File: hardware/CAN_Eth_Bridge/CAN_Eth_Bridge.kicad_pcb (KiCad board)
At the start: 2 copper layers, 22.6 x 85 mm, 72 parts, among them J101 Conn_01x05_Pin, J102 Global LV and CAN, J301 RJ45_Amphenol_RJMG1BD3B8K1ANR, Q301 MMBT5550L, Q302 MMBT5550L, SW102 SW_DIP_x06, U101 MCP2542FDxMF, U102 AP7384-50SA, U103 XMSM0G3507SDGS28R, U104 AP7381-33SA-7, U301 W5500, Y301 Crystal_GND24

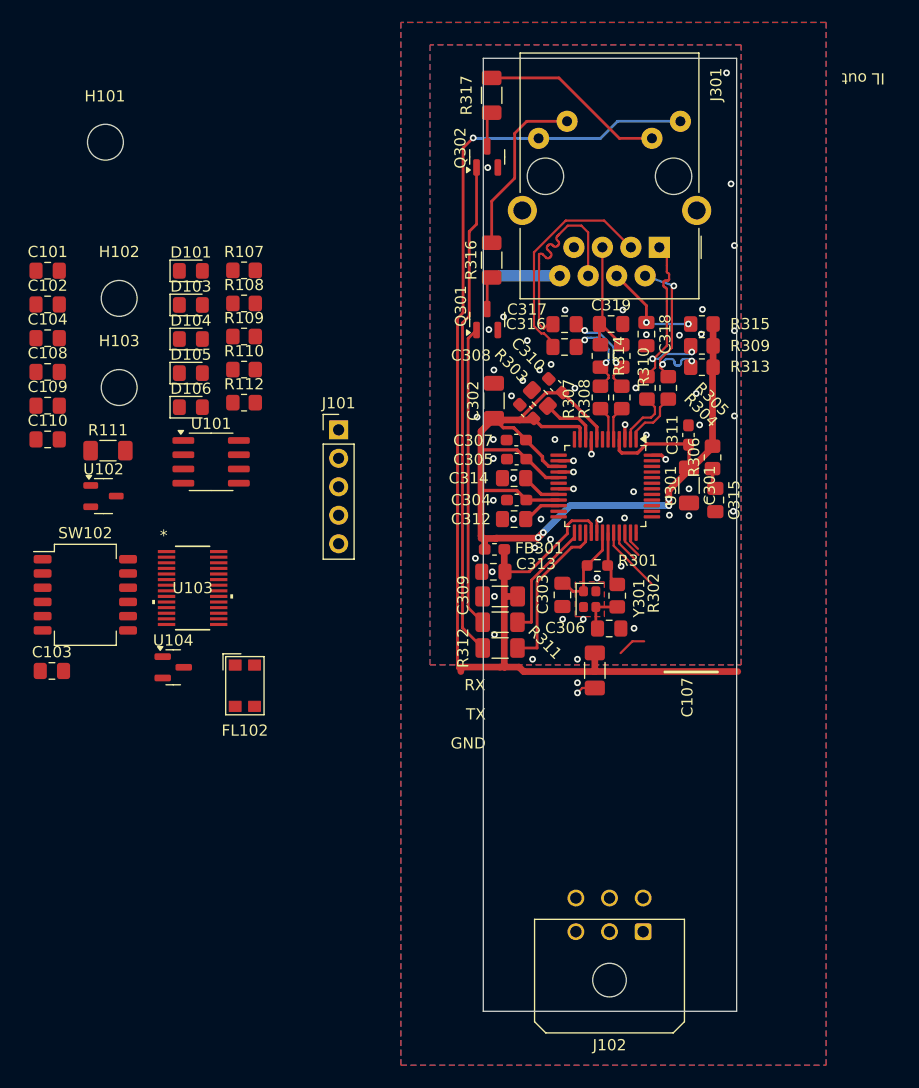
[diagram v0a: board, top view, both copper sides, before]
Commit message: hdd failure D:
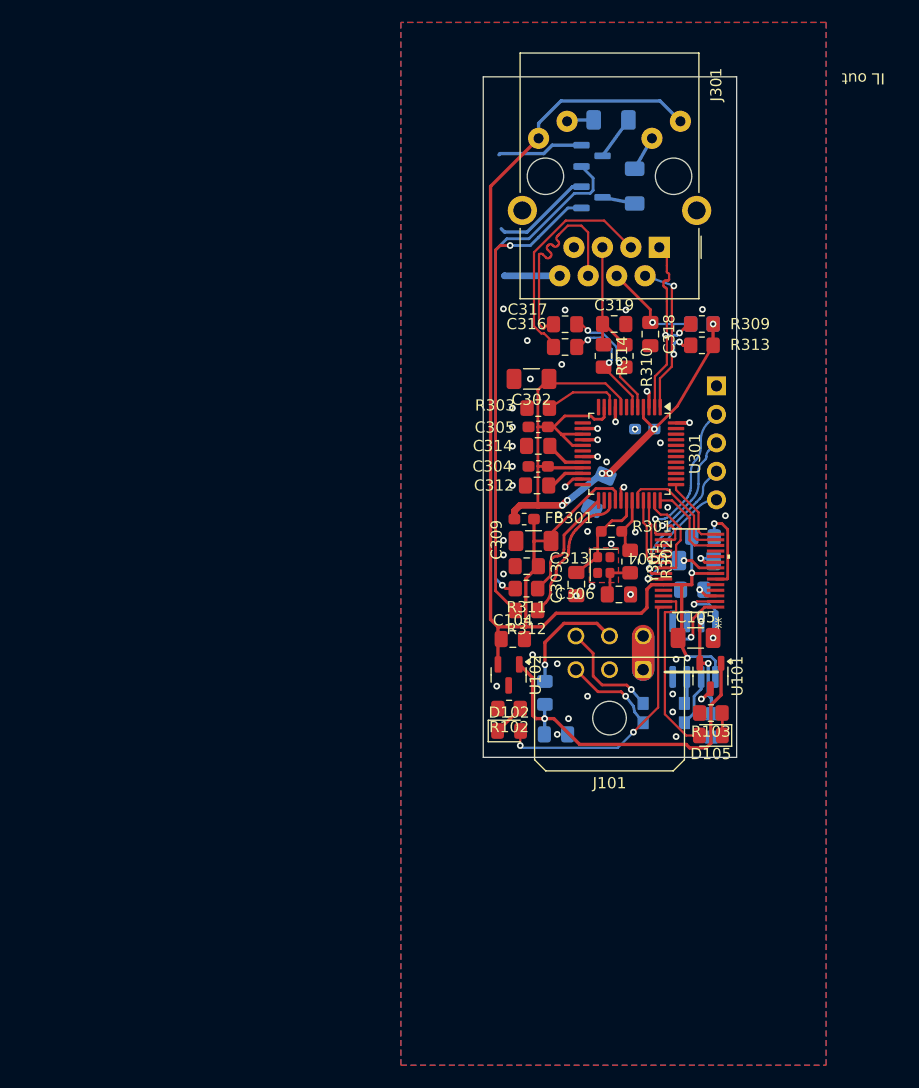
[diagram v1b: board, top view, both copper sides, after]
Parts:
- removed C102, C108, C109, C110, C315: 220n, Capacitor_SMD:C_0805_2012Metric_Pad1.18x1.45mm_HandSolder
- removed C107: 10u, Capacitor_SMD:C_1206_3216Metric_Pad1.33x1.80mm_HandSolder
- removed C307, C308, C310: 100n, Capacitor_SMD:C_0603_1608Metric_Pad1.08x0.95mm_HandSolder
- removed D103, D104: yellow, LED_SMD:LED_0805_2012Metric_Pad1.15x1.40mm_HandSolder
- removed D106: blue, LED_SMD:LED_0805_2012Metric_Pad1.15x1.40mm_HandSolder
- removed FL102: Choke_CommonMode_FerriteCore_1243, Inductor_SMD:L_CommonModeChoke_Coilcraft_1812CAN
- removed H101, H102, H103: MountingHole, MountingHole:MountingHole_3.2mm_M3
- removed R107, R108, R109: 2.4k, Resistor_SMD:R_0805_2012Metric_Pad1.20x1.40mm_HandSolder
- removed R110: 3.32k, Resistor_SMD:R_0805_2012Metric_Pad1.20x1.40mm_HandSolder
- removed R111: 100k, Resistor_SMD:R_1206_3216Metric_Pad1.30x1.75mm_HandSolder
- removed R112: 40.2k, Resistor_SMD:R_0805_2012Metric_Pad1.20x1.40mm_HandSolder
- removed R304, R305, R307, R308: 14.3, Resistor_SMD:R_0805_2012Metric_Pad1.20x1.40mm_HandSolder
- removed R306: 10, Resistor_SMD:R_0805_2012Metric_Pad1.20x1.40mm_HandSolder
- removed SW102: SW_DIP_x06, Button_Switch_SMD:SW_DIP_SPSTx06_Slide_Copal_CHS-06B_W7.62mm_P1.27mm
- added C105: 10u, Capacitor_SMD:C_1206_3216Metric_Pad1.33x1.80mm_HandSolder, F.Cu at (152.3, 111.7)
- added C106: 220n, Capacitor_SMD:C_0805_2012Metric_Pad1.18x1.45mm_HandSolder, B.Cu at (152.0, 107.4)
- added D102: green, LED_SMD:LED_0805_2012Metric_Pad1.15x1.40mm_HandSolder, F.Cu at (135.7, 120.0)
- added FL101: Choke_CommonMode_FerriteCore_1243, Inductor_SMD:L_CommonModeChoke_Coilcraft_1812CAN, B.Cu at (149.5, 118.4)
- added R102: 2.4k, Resistor_SMD:R_0805_2012Metric_Pad1.20x1.40mm_HandSolder, F.Cu at (135.7, 118.0)
- added R103: 2.4k, Resistor_SMD:R_0805_2012Metric_Pad1.20x1.40mm_HandSolder, F.Cu at (153.7, 118.4)
- added R104: 2.4k, Resistor_SMD:R_0805_2012Metric_Pad1.20x1.40mm_HandSolder, B.Cu at (153.0, 102.7)
- added R105: 100k, Resistor_SMD:R_1206_3216Metric_Pad1.30x1.75mm_HandSolder, B.Cu at (152.4, 104.8)
- C101, C103, C301, C311, D101, Q301, Q302, R315, R316, R317: moved to B.Cu
- D105: value red -> blue
- J101: value Conn_01x05_Pin -> Global LV and CAN; footprint Connector_PinHeader_2.54mm:PinHeader_1x05_P2.54mm_Vertical -> Connector_Molex:Molex_Micro-Fit_3.0_43045-0600_2x03_P3.00mm_Horizontal
- J102: value Global LV and CAN -> Conn_01x05_Pin; footprint Connector_Molex:Molex_Micro-Fit_3.0_43045-0600_2x03_P3.00mm_Horizontal -> Connector_PinHeader_2.54mm:PinHeader_1x05_P2.54mm_Vertical; moved to B.Cu
- R311, R312: value 4.99k -> 3.32k; footprint Resistor_SMD:R_1206_3216Metric_Pad1.30x1.75mm_HandSolder -> Resistor_SMD:R_0805_2012Metric_Pad1.20x1.40mm_HandSolder
- U101: value MCP2542FDxMF -> AP7384-50SA; footprint Package_SO:SOIC-8_3.9x4.9mm_P1.27mm -> Package_TO_SOT_SMD:SOT-23-3
- U102: value AP7384-50SA -> AP7381-33SA-7; footprint Package_TO_SOT_SMD:SOT-23-3 -> Package_TO_SOT_SMD:SOT-23
- U103: value XMSM0G3507SDGS28R -> MCP2542FDxMF; footprint zzLocalLibraries-Footprints:VSSOP28_DGS_TEX-M -> Package_SO:SOIC-8_3.9x4.9mm_P1.27mm; moved to B.Cu
- U104: value AP7381-33SA-7 -> XMSM0G3507SDGS28R; footprint Package_TO_SOT_SMD:SOT-23 -> zzLocalLibraries-Footprints:VSSOP28_DGS_TEX-M
- moved C101 61.4 mm to (139.9, 120.3)
- moved C103 59.0 mm to (153.8, 119.5), turned to -90 degrees
- moved D105 56.5 mm to (153.7, 120.4), turned to 180 degrees
- moved C104 49.4 mm to (136.0, 111.8)
- moved D101 49.1 mm to (138.9, 116.6), turned to 90 degrees
- moved J102 49.1 mm to (154.2, 89.2)
- moved U101 48.5 mm to (153.7, 115.1), turned to -90 degrees
- moved U104 46.9 mm to (151.8, 105.7), turned to 180 degrees
- moved U103 45.1 mm to (152.2, 112.7), turned to -90 degrees
- moved U102 39.5 mm to (135.7, 115.0), turned to -90 degrees
- moved J101 34.6 mm to (147.7, 114.5), turned to 180 degrees
- moved Q301 17.3 mm to (143.1, 68.7), turned to 0 degrees
- moved R316 16.4 mm to (144.8, 65.5), turned to 180 degrees
- moved R317 15.1 mm to (146.9, 71.4)
- moved Q302 10.0 mm to (143.1, 72.4), turned to 0 degrees
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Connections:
- C101 pad 1: +3.3V -> Net-(D101-K)
- C103 pad 1: Net-(D101-K) -> +5V
- C104 pad 1: +5V -> +3.3V
- C316 pad 1: /Ethernet/RX_1+ -> /Ethernet/RX+
- C317 pad 1: /Ethernet/RX_1- -> /Ethernet/RX-
- D105 pad 1: GND -> Net-(D105-K)
- D105 pad 2: Net-(D105-A) -> /led.sched
- J101 pad 1: GND -> /G_IL+
- J101 pad 2: /prog.uart_ui_rx -> GND
- J101 pad 3: /prog.uart_ui_tx -> /G_CAN-
- J101 pad 4: /prog.SWDIO -> /G_IL+
- J101 pad 5: /prog.SWCLK -> /GLV+
- J102 pad 1: /G_IL+ -> GND
- J102 pad 2: GND -> /prog.uart_ui_tx
- J102 pad 3: /G_CAN- -> /prog.uart_ui_rx
- J102 pad 4: /G_IL+ -> /prog.SWDIO
- J102 pad 5: /GLV+ -> /prog.SWCLK
- R310 pad 2: /Ethernet/RX_1- -> /Ethernet/RX-
- R314 pad 2: /Ethernet/RX_1+ -> /Ethernet/RX+
- U101 pad 1: /can.tx -> Net-(D101-K)
- U101 pad 2: GND -> +5V
- U101 pad 3: +5V -> GND
- U102 pad 2: +5V -> +3.3V
- U103 pad 1: unconnected-(U103-PA26/A0_1-Pad1) -> /can.tx
- U103 pad 2: unconnected-(U103-PA27/RTC_OUT/A0_0-Pad2) -> GND
- U103 pad 3: /vcore -> +5V
- U103 pad 4: unconnected-(U103-PA0-Pad4) -> /can.rx
- U103 pad 5: unconnected-(U103-PA1-Pad5) -> +3.3V
- U103 pad 7: +3.3V -> Net-(U103-CANH)
- U104 pad 1: Net-(D101-K) -> /can.tx
- U104 pad 2: +3.3V -> /can.rx
- U104 pad 3: GND -> /vcore
- U301 pad 1: /Ethernet/TX- -> /Ethernet/TD-
- U301 pad 2: /Ethernet/TX+ -> /Ethernet/TD+
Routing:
- net /Ethernet/+3.3VA: track 102.0 -> 66.8 mm, vias 4 -> 6
- net Net-(D101-K): track 0.00 -> 32.6 mm, vias 0 -> 1
- net /led.i1: track 0.00 -> 24.5 mm, vias 0 -> 2
- net GND: track 16.7 -> 37.5 mm, vias 61 -> 48
- net Net-(Q301-B): track 26.9 -> 44.9 mm, vias 0 -> 1
- net /led.sched: track 0.00 -> 16.0 mm
- net /prog.uart_ui_tx: track 0.00 -> 13.8 mm, vias 0 -> 1
- net Net-(J301-PadL3): track 16.5 -> 3.12 mm
- net Net-(J301-PadL2): track 15.7 -> 2.42 mm
- net /prog.uart_ui_rx: track 0.00 -> 12.5 mm, vias 0 -> 1
- net /prog.SWDIO: track 0.00 -> 12.4 mm, vias 0 -> 1
- net /prog.SWCLK: track 0.00 -> 11.2 mm, vias 0 -> 1
- net /GLV+: track 0.00 -> 10.4 mm, vias 0 -> 1
- net /G_CAN+: track 0.00 -> 9.73 mm, vias 0 -> 1
- net +5V: track 0.00 -> 9.16 mm, vias 0 -> 2
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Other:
- board size 22.6 x 85 mm -> 22.6 x 60.7 mm
- board text added: "CAN-Ethernet bridge github.com/Gregification/BeeMS/ 2/8/2026 - pinning & design:"
- board text added: "SWCLK"
- board text added: "SWDIO"
- board text added: "hope and dreams kind of routing"
- board text removed: "5V out"
- board text removed: "E27 accumulator LV-ish garage top view"
- board text removed: "ETH"
- board text removed: "GLV"
- board text removed: "HRLV"
- board text removed: "HV cross path. AIRs(TSBPIRs?), main fuse,"
- board text removed: "LV connectors somewhere over here"
- board text removed: "MCHS"
- board text removed: "Master Board A 1.1 (testing use only) github.com/Gregification/BeeMS/ 1/13/2025 - pinning & hardware info: {dblquote}/hardware/MasterBoard_A/meta.xlsx{dblquote} - software: {dblquote}/MB_MSPM0G3507_A{dblquote} - no hardware watchdog - no PWM bank"
- board text removed: "Master Board go about here"
- board text removed: "PWM SB1"
- board text removed: "cut out to segments below"
- board text removed: "hope and dreams kind of wiring"
- board text removed: "impercise"
- board text removed: "not to scale"
- board text removed: "percise"
- board text removed: "we dont talk about this routing"
